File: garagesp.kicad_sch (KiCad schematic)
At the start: 43 parts, among them J1 USB_C_Receptacle_USB2.0_14P, J2 AHT21, J3 DOOR CTL, J4 DOOR SW, K1 SANYOU_SRD_Form_A, Q1 SS8050, Q2 SS8050, U1 ESP32-C3-WROOM-02, U2 AMS1117-3.3, U3 USBLC6-2SC6, U4 PC817

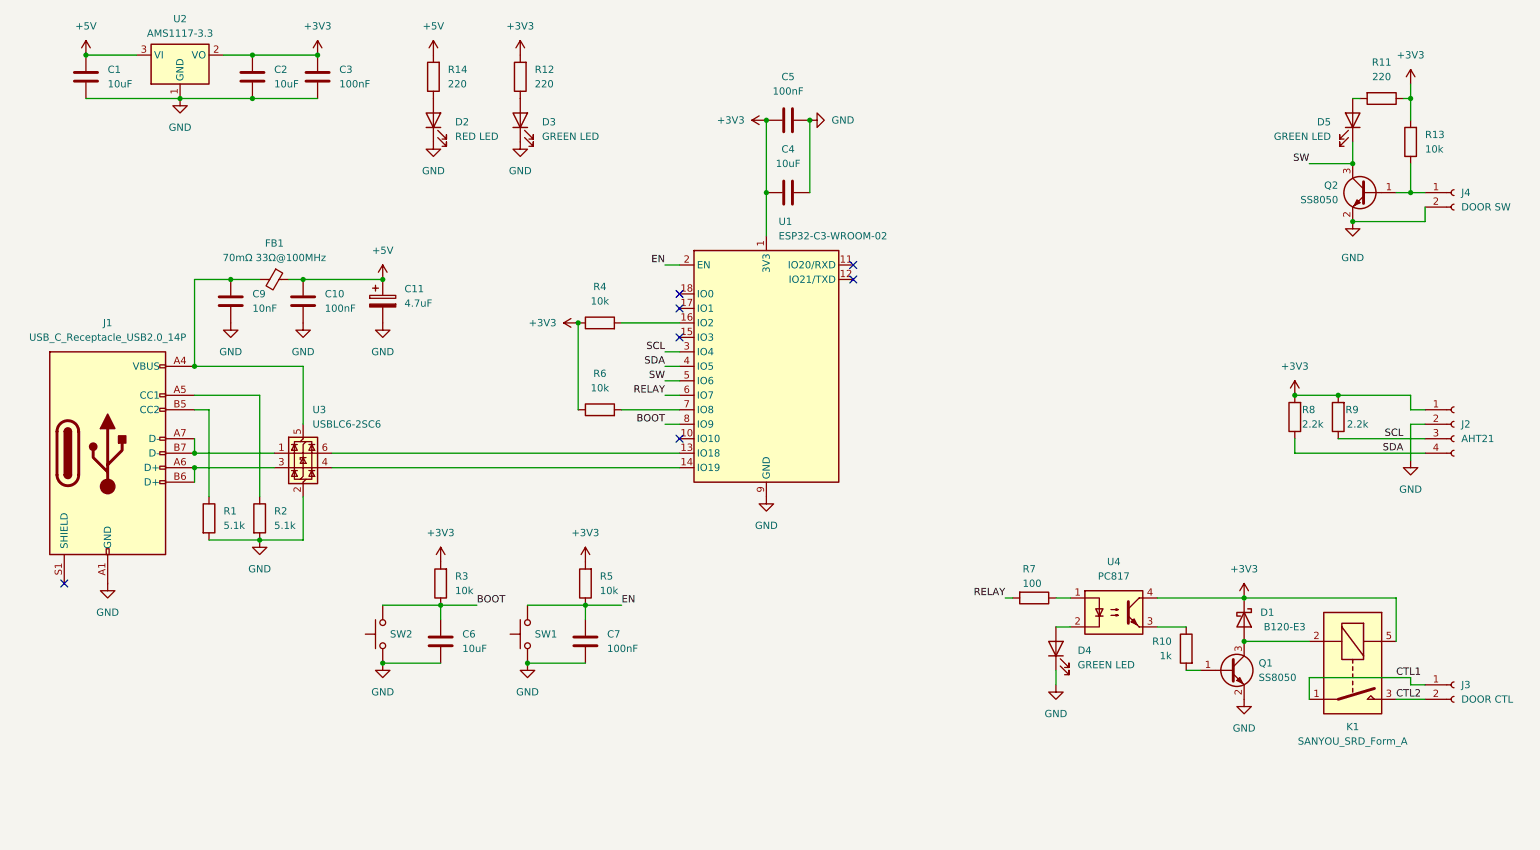
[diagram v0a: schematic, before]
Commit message: I like this but want to invert my input LEDs
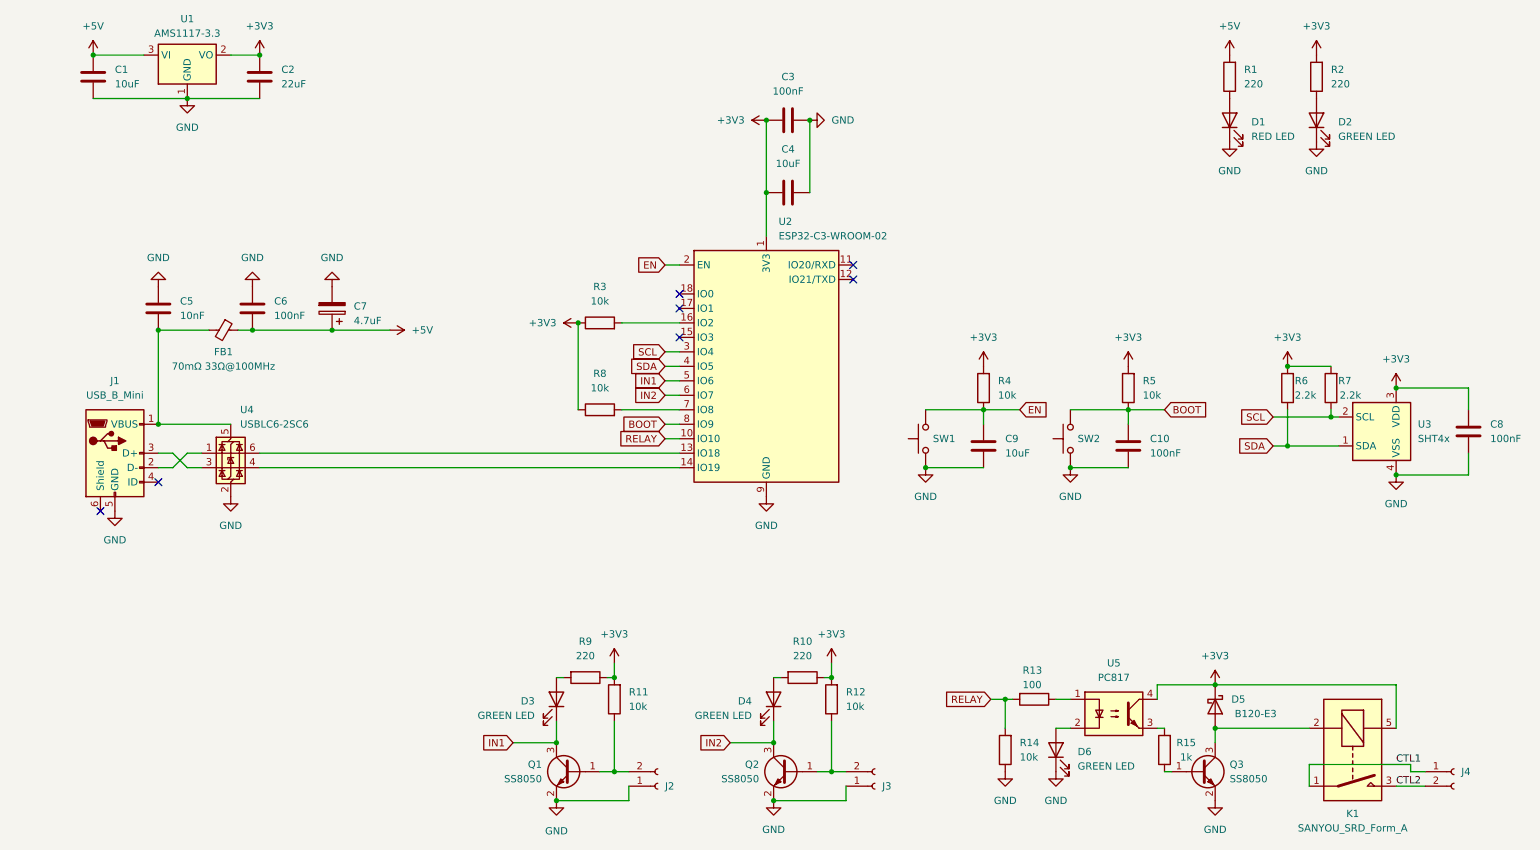
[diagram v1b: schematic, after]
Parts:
- removed C3: 100nF, Capacitor_SMD:C_0603_1608Metric_Pad1.08x0.95mm_HandSolder, symbol Device:C
- removed J1: USB_C_Receptacle_USB2.0_14P, Connector_USB:USB_C_Receptacle_HCTL_HC-TYPE-C-16P-01A, symbol Connector:USB_C_Receptacle_USB2.0_14P
- removed J2: AHT21, Connector_PinSocket_2.54mm:PinSocket_1x04_P2.54mm_Vertical, symbol Connector:Conn_01x04_Socket
- removed R1, R2: 5.1k, Resistor_SMD:R_0603_1608Metric_Pad0.98x0.95mm_HandSolder, symbol Device:R
- removed R10: 1k, Resistor_SMD:R_0603_1608Metric_Pad0.98x0.95mm_HandSolder, symbol Device:R
- added C8: 100nF, Capacitor_SMD:C_0402_1005Metric_Pad0.74x0.62mm_HandSolder, symbol Device:C
- added D3: GREEN LED, LED_SMD:LED_0603_1608Metric_Pad1.05x0.95mm_HandSolder, symbol Device:LED
- added J1: USB_B_Mini, Connector_USB:USB_Mini-B_Lumberg_2486_01_Horizontal, symbol Connector:USB_B_Mini
- added J2: ~, Connector_Molex:Molex_Micro-Fit_3.0_43650-0200_1x02_P3.00mm_Horizontal, symbol Connector:Conn_01x02_Socket
- added Q1: SS8050, Package_TO_SOT_SMD:SOT-23, symbol Transistor_BJT:SS8050
- added R11, R14: 10k, Resistor_SMD:R_0603_1608Metric_Pad0.98x0.95mm_HandSolder, symbol Device:R
- added R15: 1k, Resistor_SMD:R_0603_1608Metric_Pad0.98x0.95mm_HandSolder, symbol Device:R
- added R9: 220, Resistor_SMD:R_0603_1608Metric_Pad0.98x0.95mm_HandSolder, symbol Device:R
- added U3: SHT4x, Sensor_Humidity:Sensirion_DFN-4_1.5x1.5mm_P0.8mm_SHT4x_NoCentralPad, symbol Sensor_Humidity:SHT4x
- C2: value 10uF -> 22uF; LCSC C19702 -> C59461
- J3: renamed from J4; value DOOR SW -> ~; LCSC C192562 -> C122431
- J4: renamed from J3; value DOOR CTL -> ~; LCSC C192562 -> C122431
- renumbered C7 to C10, C5 to C3, C9 to C5, C10 to C6, C11 to C7, C6 to C9, D2 to D1, D3 to D2, D5 to D4, D1 to D5, D4 to D6, Q1 to Q3, R14 to R1, R11 to R10, R13 to R12, R7 to R13, R12 to R2, R4 to R3, R3 to R4, R8 to R6, R9 to R7, R6 to R8, SW2 to SW1, SW1 to SW2, U2 to U1, U1 to U2, U3 to U4, U4 to U5
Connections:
- net +3V3: now also C8.2, R11.2, R9.1, U3.3 (VDD)
- net BOOT: now also C10.2, R5.1, SW2.2; no longer C9.1, R4.1, SW1.2
- net EN: now also C9.1, R4.1, SW1.2; no longer C10.2, R5.1, SW2.2
- net GND: now also J3.1 (Pin_1), C8.1, J1.5 (GND), J2.1 (Pin_1), Q1.2 (E), R14.1, U3.4 (VSS); no longer J3.2 (Pin_2)
- net RELAY: now also U2.10 (IO10), R14.2; no longer U2.6 (IO7)
- net SCL: now also U3.2 (SCL)
- net SDA: now also U3.1 (SDA)
- net at Q2.1 (B), R12.1: now also J3.2 (Pin_2); no longer J3.1 (Pin_1)
- net at Q3.1 (B): now also R15.1
- net at C5.1, FB1.2, U4.5 (VBUS): now also J1.1 (VBUS)
- net at U5.3: now also R15.2
- net SW renamed IN2
- net IN2: now also U2.6 (IO7); no longer U2.5 (IO6)
- new net: J2.2 (Pin_2), Q1.1 (B), R11.1
- new net: D3.2 (A), R9.2
- new net IN1: D3.1 (K), Q1.3 (C), U2.5 (IO6)
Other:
- moved on the sheet: C1, C10, C2, C5, C6, C7, C9, D1, D2, D4, D5, D6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
